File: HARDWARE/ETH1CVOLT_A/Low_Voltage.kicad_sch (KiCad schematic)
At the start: 63 parts, among them J5 1715734, Q3 FZT849, U10 TSR0.5-2490, U11 LT8330_S6, U12 LT8330_S6, U15 TPS7A39, U16 ADP7142ARDZ-5.0, U17 ADP7142ARDZ-3.3

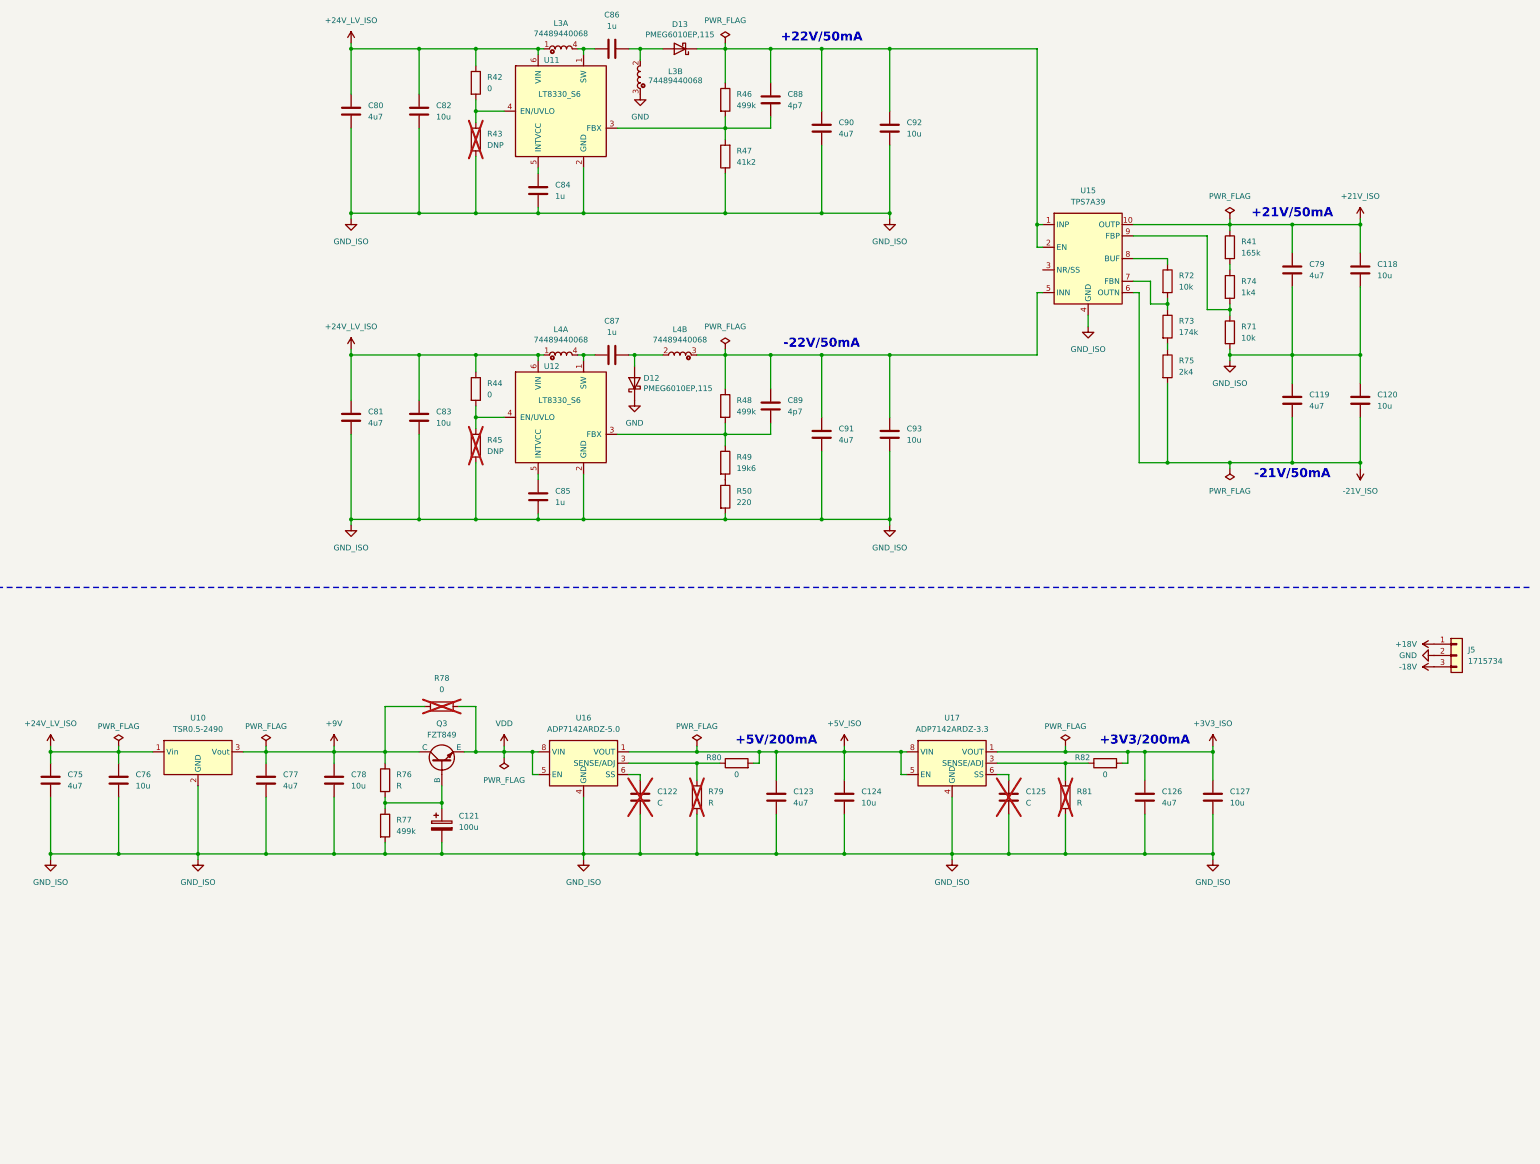
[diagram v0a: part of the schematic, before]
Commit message: Development
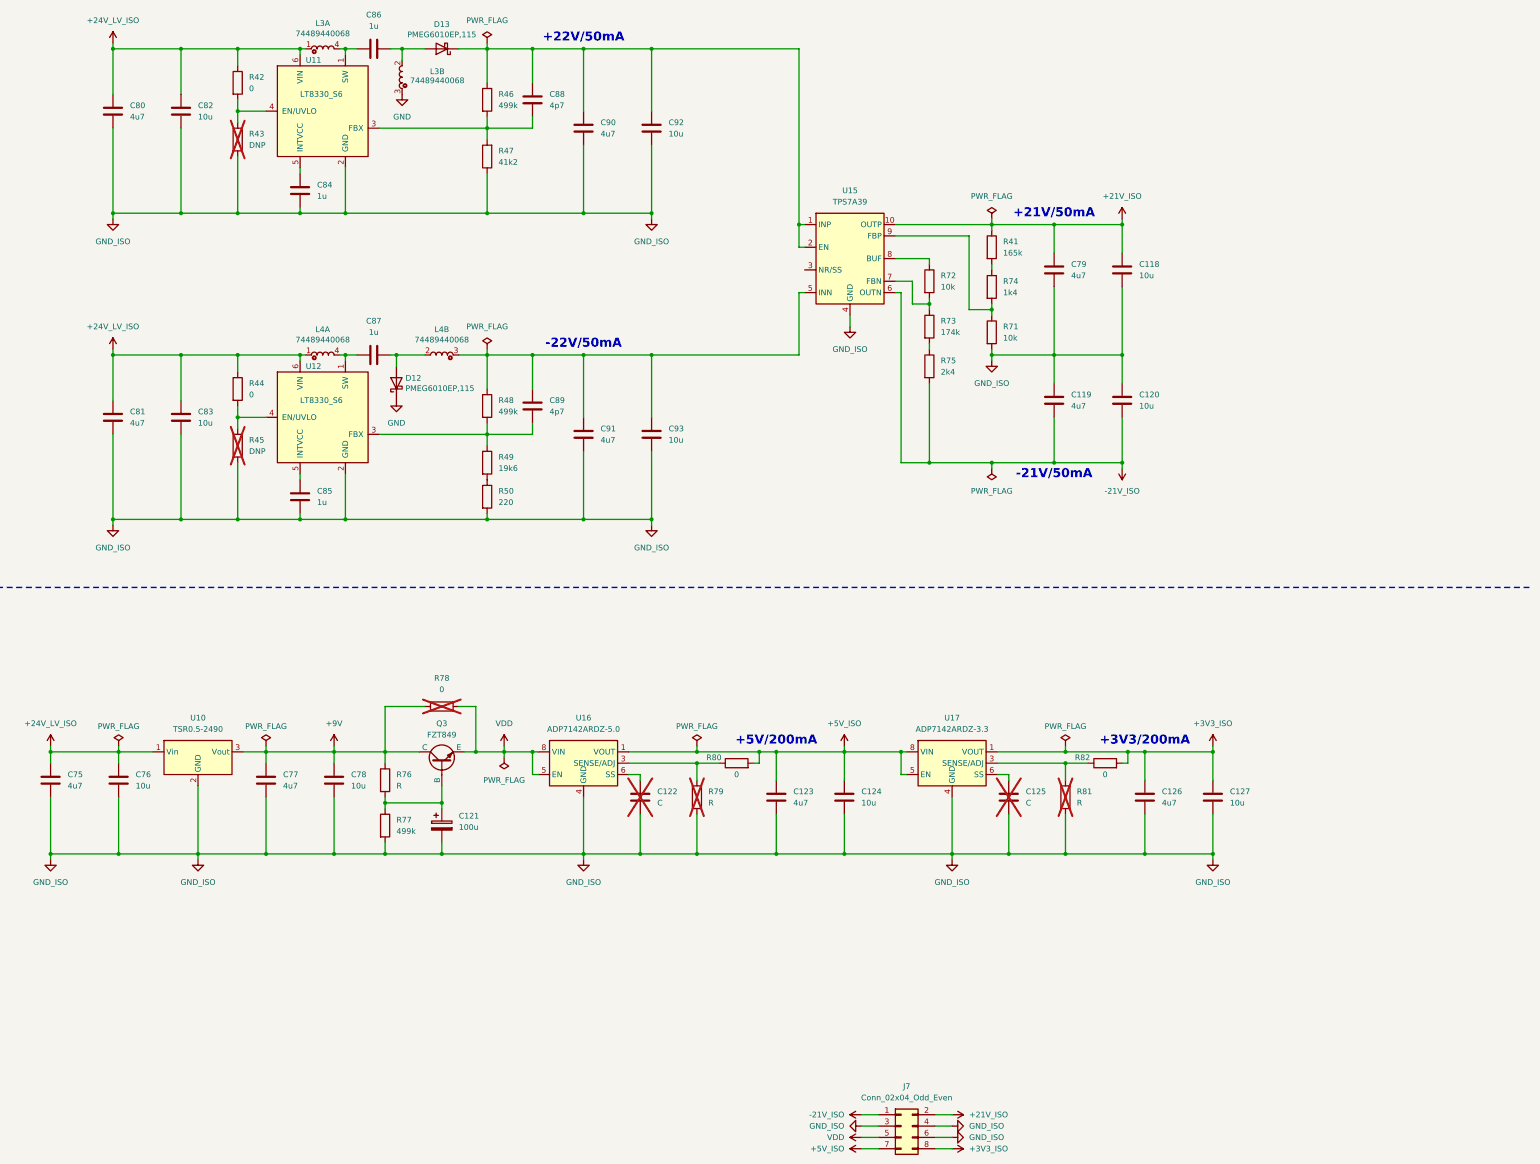
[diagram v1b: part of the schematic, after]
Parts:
- removed J5: 1715734, TerminalBlock_Phoenix:TerminalBlock_Phoenix_MKDS-1,5-3-5.08_1x03_P5.08mm_Horizontal, symbol Connector_Generic:Conn_01x03
- added J7: Conn_02x04_Odd_Even, Connector_PinSocket_2.54mm:PinSocket_2x04_P2.54mm_Vertical_SMD, symbol Connector_Generic:Conn_02x04_Odd_Even
- C84, C85, C86, C87, C88, C89: footprint (none) -> Capacitor_SMD:C_0603_1608Metric_Pad1.08x0.95mm_HandSolder
- L3, L4: footprint UCC25800:74489440068 -> ETH1CVOLT_A:74489440068
- R41, R42, R43, R44, R45, R46, R47, R48, R49, R50, R71, R72, R73, R74, R75, R76, R77, R80, R82: footprint (none) -> Resistor_SMD:R_0603_1608Metric_Pad0.98x0.95mm_HandSolder
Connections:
- net +21V_ISO: now also J7.2 (Pin_2)
- net +3V3_ISO: now also J7.8 (Pin_8)
- net +5V_ISO: now also J7.7 (Pin_7)
- net -21V_ISO: now also J7.1 (Pin_1)
- net GND_ISO: now also J7.3 (Pin_3), J7.4 (Pin_4), J7.6 (Pin_6)
- net VDD: now also J7.5 (Pin_5)
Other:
- moved on the sheet: C118, C119, C120, C79, C80, C81, C82, C83, C84, C85, C86, C87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
